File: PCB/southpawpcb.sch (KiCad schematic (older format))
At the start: 158 parts, among them K1 KEYSW, K10 KEYSW, K11 KEYSW, K12 KEYSW, K13 KEYSW, K14 KEYSW, K15 KEYSW, K16 KEYSW, K17 KEYSW, K18 KEYSW, K19 KEYSW, K2 KEYSW, K20 KEYSW, K21 KEYSW, K22 KEYSW, K23 KEYSW, K24 KEYSW, K25 KEYSW, K26 KEYSW, K27 KEYSW, K28 KEYSW, K29 KEYSW, K3 KEYSW, K30 KEYSW, K31 KEYSW, K32 KEYSW, K33 KEYSW, K34 KEYSW, K35 KEYSW, K36 KEYSW, K37 KEYSW, K38 KEYSW, K39 KEYSW, K4 KEYSW, K40 KEYSW, K41 KEYSW, K42 KEYSW, K43 KEYSW, K44 KEYSW, K45 KEYSW, K46 KEYSW, K47 KEYSW, K48 KEYSW, K49 KEYSW, K5 KEYSW, K50 KEYSW, K51 KEYSW, K52 KEYSW, K53 KEYSW, K54 KEYSW, K55 KEYSW, K56 KEYSW, K57 KEYSW, K58 KEYSW, K59 KEYSW, K6 KEYSW, K60 KEYSW, K61 KEYSW, K62 KEYSW, K63 KEYSW, K64 KEYSW, K65 KEYSW, K66 KEYSW, K67 KEYSW, K68 KEYSW, K69 KEYSW, K7 KEYSW, K70 KEYSW, K71 KEYSW, K72 KEYSW, K73 KEYSW, K74 KEYSW, K75 KEYSW, K76 KEYSW, K77 KEYSW, K78 KEYSW, K8 KEYSW, K9 KEYSW, SW1 Reset, U1 ProMicro

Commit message: attempt at retracing
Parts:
- K1, K10, K11, K12, K13, K14, K15, K16, K17, K19, K2, K20, K21, K24, K25, K26, K27, K28, K29, K3, K30, K31, K32, K33, K34, K35, K37, K38, K39, K4, K41, K42, K43, K44, K45, K46, K47, K48, K49, K5, K50, K51, K53, K54, K55, K58, K59, K6, K60, K61, K62, K63, K64, K65, K66, K67, K7, K70, K8, K9: footprint MX/Alps_Hybrid:MX-1U-NoLED -> MX_Only:MXOnly-1U-Hotswap; symbol Keyboard_Parts1:KEYSW -> MX_Alps_Hybrid:MX-NoLED
- K18, K22, K56, K69: footprint MX/Alps_Hybrid:MX-2U-NoLED -> MX_Only:MXOnly-2U-Hotswap; symbol Keyboard_Parts1:KEYSW -> MX_Alps_Hybrid:MX-NoLED
- K23, K36: footprint MX/Alps_Hybrid:MX-1.5U-NoLED -> MX_Only:MXOnly-1.5U-Hotswap; symbol Keyboard_Parts1:KEYSW -> MX_Alps_Hybrid:MX-NoLED
- K40: footprint MX/Alps_Hybrid:MX-1.75U-NoLED -> MX_Only:MXOnly-1.75U-Hotswap; symbol Keyboard_Parts1:KEYSW -> MX_Alps_Hybrid:MX-NoLED
- K52, K57: footprint MX/Alps_Hybrid:MX-2.25U-NoLED -> MX_Only:MXOnly-2.25U-Hotswap; symbol Keyboard_Parts1:KEYSW -> MX_Alps_Hybrid:MX-NoLED
- K68: footprint MX/Alps_Hybrid:MX-2.75U-NoLED -> MX_Only:MXOnly-2.75U-Hotswap; symbol Keyboard_Parts1:KEYSW -> MX_Alps_Hybrid:MX-NoLED
- K71, K72, K73, K75, K76, K77, K78: footprint MX/Alps_Hybrid:MX-1.25U-NoLED -> MX_Only:MXOnly-1.25U-Hotswap; symbol Keyboard_Parts1:KEYSW -> MX_Alps_Hybrid:MX-NoLED
- K74: footprint MX/Alps_Hybrid:MX-6.25U-NoLED -> MX_Only:MXOnly-6.25U-Hotswap; symbol Keyboard_Parts1:KEYSW -> MX_Alps_Hybrid:MX-NoLED
- SW1: symbol Keyboard_Parts1:SW_PUSH -> Switch:SW_Push
- U1: footprint Pro_Micro:ProMicro -> promicro:ProMicro; symbol Pro_Micro:ProMicro -> promicro:ProMicro
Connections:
- wire segments 187 -> 118

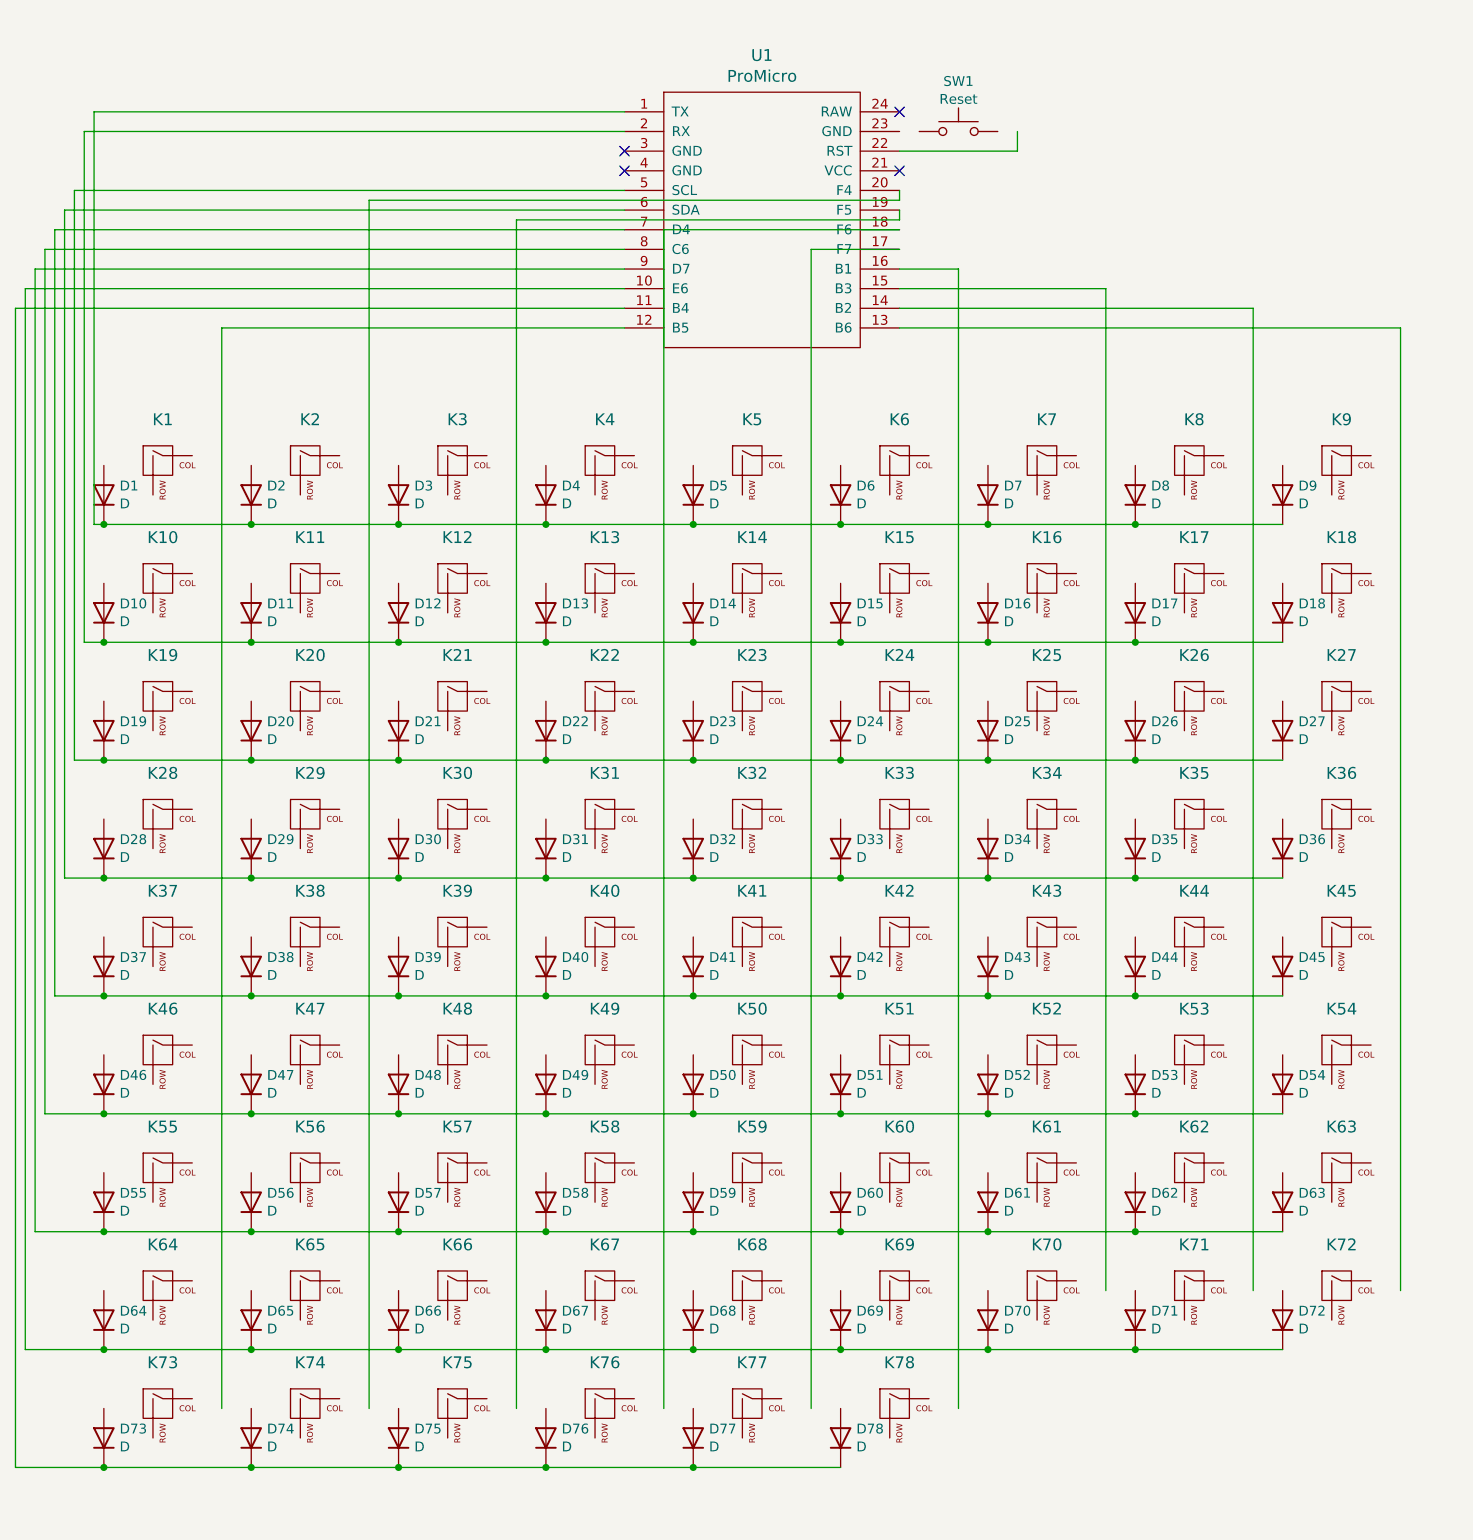
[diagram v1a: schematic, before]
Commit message: all routed
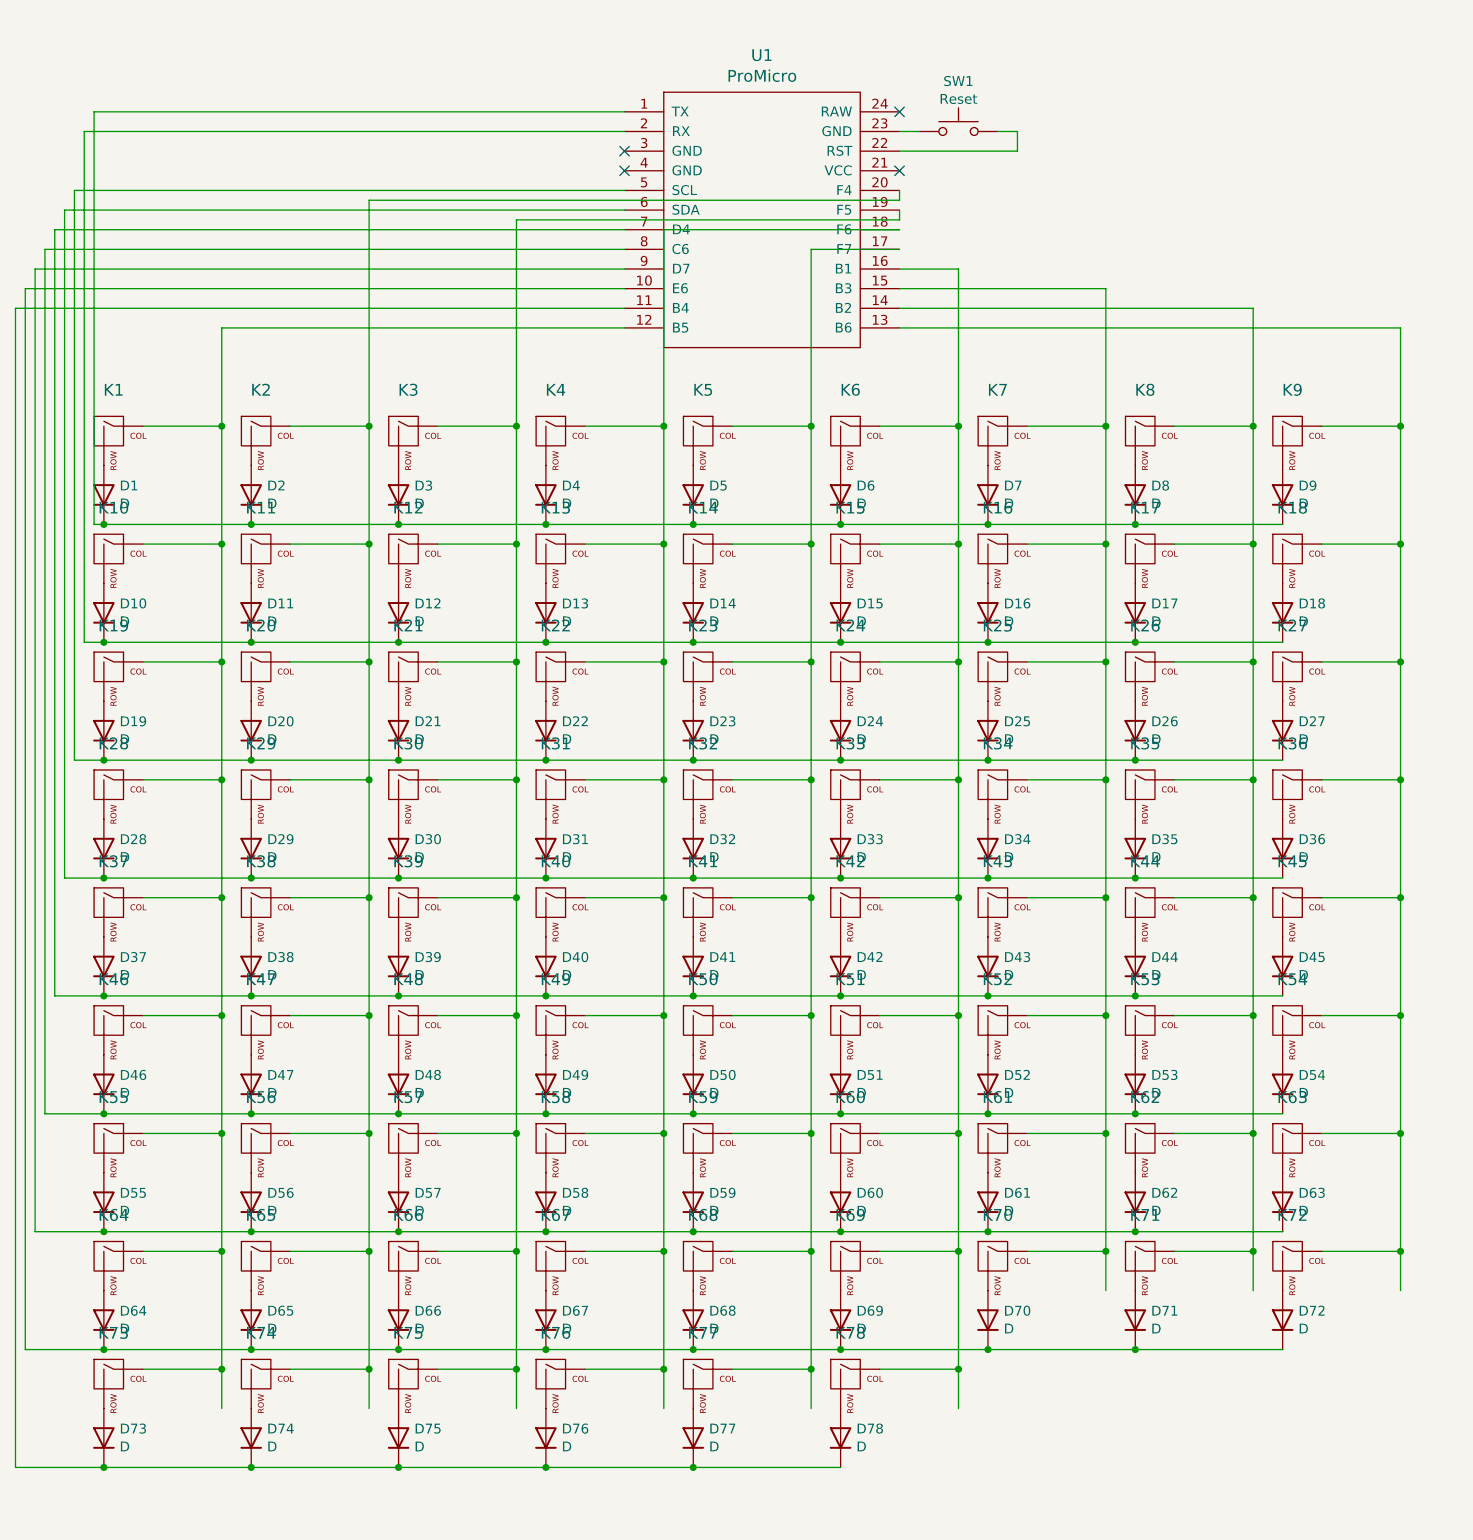
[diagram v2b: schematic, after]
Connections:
- wire segments 118 -> 276
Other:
- moved on the sheet: K1, K10, K11, K12, K13, K14, K15, K16, K17, K18, K19, K2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
